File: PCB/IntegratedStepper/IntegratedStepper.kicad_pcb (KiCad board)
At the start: 4 copper layers, 57 x 42.5 mm, 81 parts, among them CN1 PJ-35825, CN2 PJ-35825, IC2 SN65HVD230DR, IC3 LMR38020FSQDDARQ1, IC4 DRV8243HQRXYRQ1, IC5 DRV8243HQRXYRQ1, J3 Screw_Terminal_01x02, J4 Screw_Terminal_01x02, J5 Conn_01x05_Socket, Q1 SS8050-G, Q2 SS8050-G, U1 ESP32-WROOM-32E, U2 AS5048A, U3 CP2102N-Axx-xQFN28, U4 XT30PW-F, U5 XT30PW-F

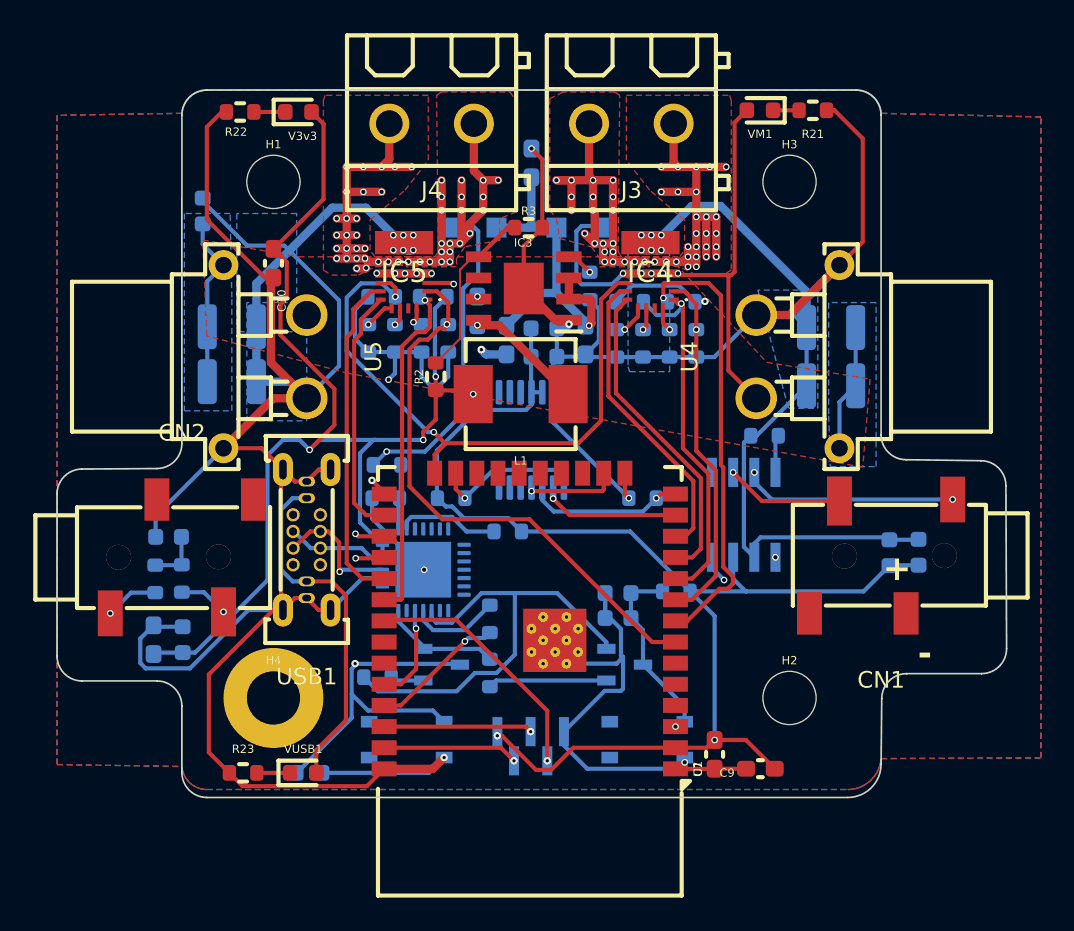
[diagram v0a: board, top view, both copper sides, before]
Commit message: Update final layout, replace CAN w/ JST
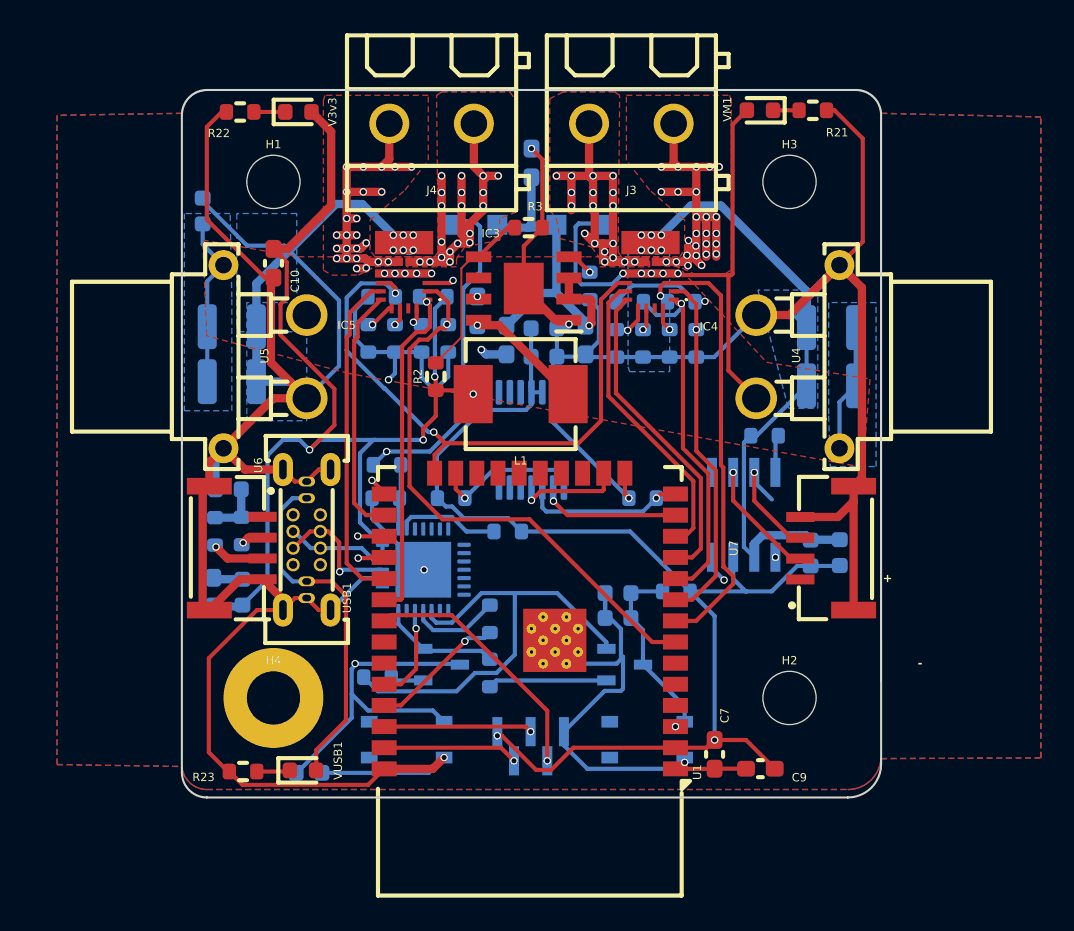
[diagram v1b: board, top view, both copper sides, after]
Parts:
- removed CN1, CN2: PJ-35825, easyeda2kicad:AUDIO-SMD_PJ-35825
- added U6: SM04B-GHS-TB(LF)(SN), easyeda2kicad:CONN-SMD_4P-P1.25_SM04B-GHS-TB-LF-SN, F.Cu at (103.2, 127.5)
- added U7: SM04B-GHS-TB(LF)(SN), easyeda2kicad:CONN-SMD_4P-P1.25_SM04B-GHS-TB-LF-SN, F.Cu at (138.8, 127.5)
- R1, R13, R14: value 10k -> 8.2k
- R15, R16, R_DRV1, R_SLEEP1, R_nFAULT_1, R_nFAULT_2: value 2k -> 8.2k
- R21: value 10K -> 8.2k
- moved C13 4.73 mm to (137.8, 127.8)
- moved C18 4.73 mm to (139.5, 127.8)
- moved C15 4.59 mm to (102.8, 124.0)
- moved C19 4.59 mm to (103.6, 130.1)
- moved C8 4.59 mm to (101.9, 130.1)
- moved R7 4.59 mm to (103.6, 126.5)
- moved R8 4.59 mm to (102.0, 126.5)
- moved D2 0.18 mm to (117.5, 108.1)
- moved D1 0.17 mm to (123.9, 108.1)
- moved VUSB1 0.15 mm to (107.3, 140.8)
- moved R23 0.08 mm to (103.7, 140.9)
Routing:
- net CANL: track 60.7 -> 48.5 mm, vias 3 -> 2
- net 3V3_VCC: track 171.7 -> 162.9 mm
- net CANH: track 50.9 -> 44.1 mm
- net GND: track 353.6 -> 357.8 mm
- net /DRV8844/OUT1: track 23.8 -> 24.3 mm, vias 21 -> 18
- net /DRV8844/OUT3: track 21.6 -> 21.2 mm, vias 27 -> 24
- net /DRV8844/OUT4: track 21.2 -> 21.5 mm, vias 21 -> 19
- net /DRV8844/OUT2: track 23.0 -> 22.8 mm, vias 27 -> 26
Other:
- board size 57 x 42.5 mm -> 42 x 42.5 mm
- board text added: "v2.0, 5/2024"
- board text removed: "v1.0, 3/2024"
